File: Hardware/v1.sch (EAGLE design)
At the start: 77 parts, among them IC1 LM324D, IC2 m328p, IC3 REG1117, J1 22-27-2061-06, J2 22-27-2021-02, J3 22-27-2021-02, J4 22-27-2031-03, J5 22-27-2041-04, Q1 BSS123, Q2 BSS123, Q3 BSS123, Q5 BSS123

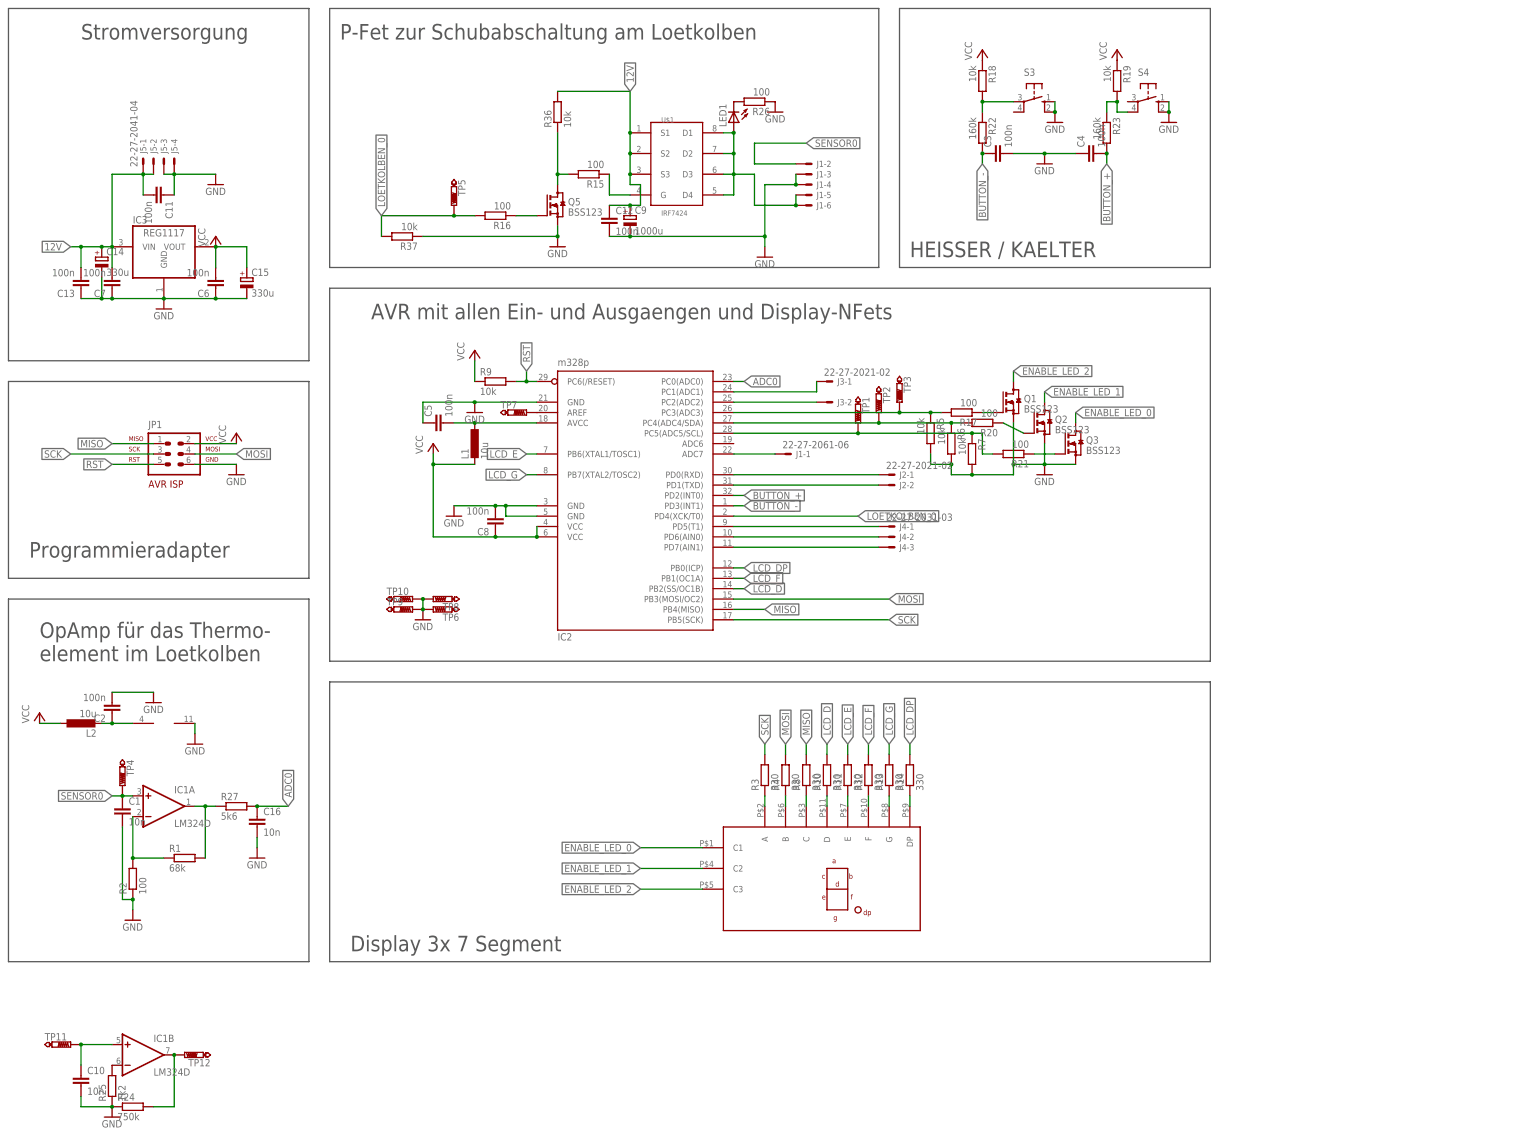
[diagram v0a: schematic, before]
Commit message: latest version with some updates
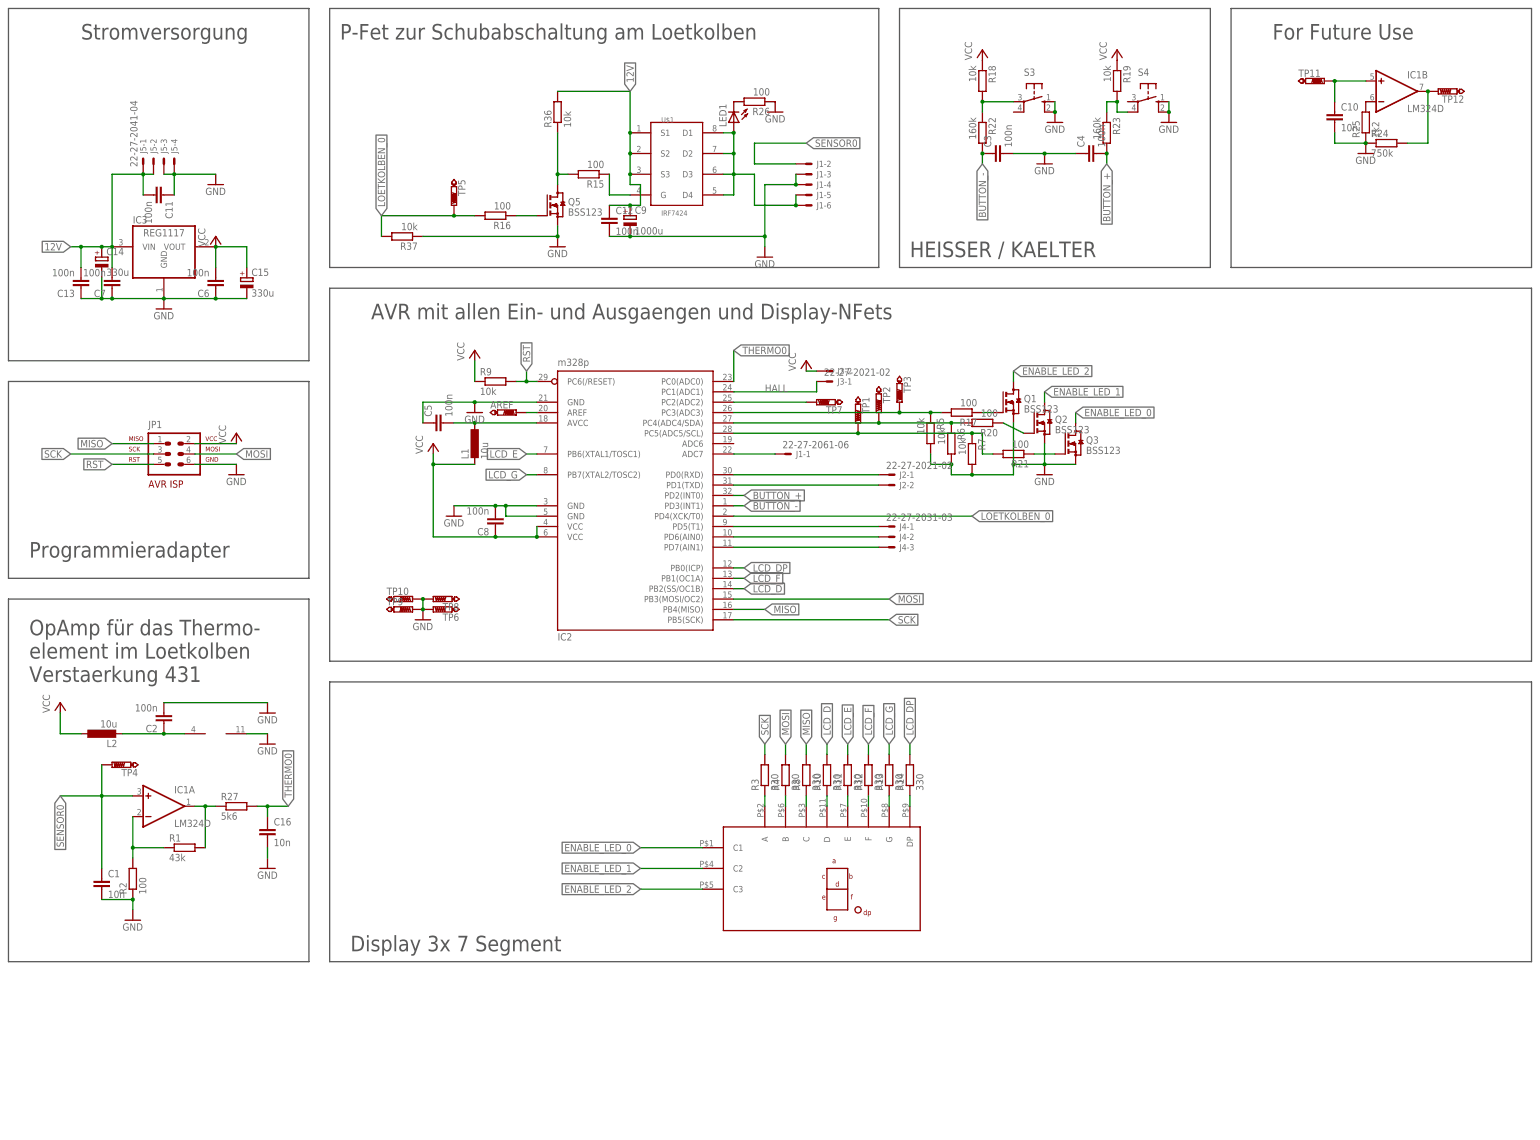
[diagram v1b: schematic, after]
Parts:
- added AREF: PTR1B1,27, testpad:PTR1B1,27
- R1: value 68k -> 43k
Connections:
- net ADC0 renamed THERMO0
- net ADC1 renamed HALL
- removed net N$24: IC2.AREF, TP7.TP
- new net AREF: AREF.TP, IC2.AREF
- net ADC2: now also TP7.TP; no longer J3-2.S
- net VCC: now also J3-2.S
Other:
- note added: "For Future Use"
- note added: "OpAmp für das Thermo- element im Loetkolben Verstaerkung 431"
- note removed: "OpAmp für das Thermo- element im Loetkolben"
- moved on the sheet: C1, C10, C16, C2, IC1B, J3-2, L2, R1, R24, R25, TP11, TP12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
